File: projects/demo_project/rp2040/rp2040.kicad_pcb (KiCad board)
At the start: 2 copper layers, 30 x 60 mm, 39 parts, among them J1 1x20, J2 TC2030-IDC-NL, J3 USB_C_Receptacle_Molex_216990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, J4 1x20, SW1 PTS815, SW2 PTS815, U1 RP2040, U2 W25Q16JV, U3 TPS63051, U5 SHT40-AD1B, Y1 CSTNE12M0GH5L000R0

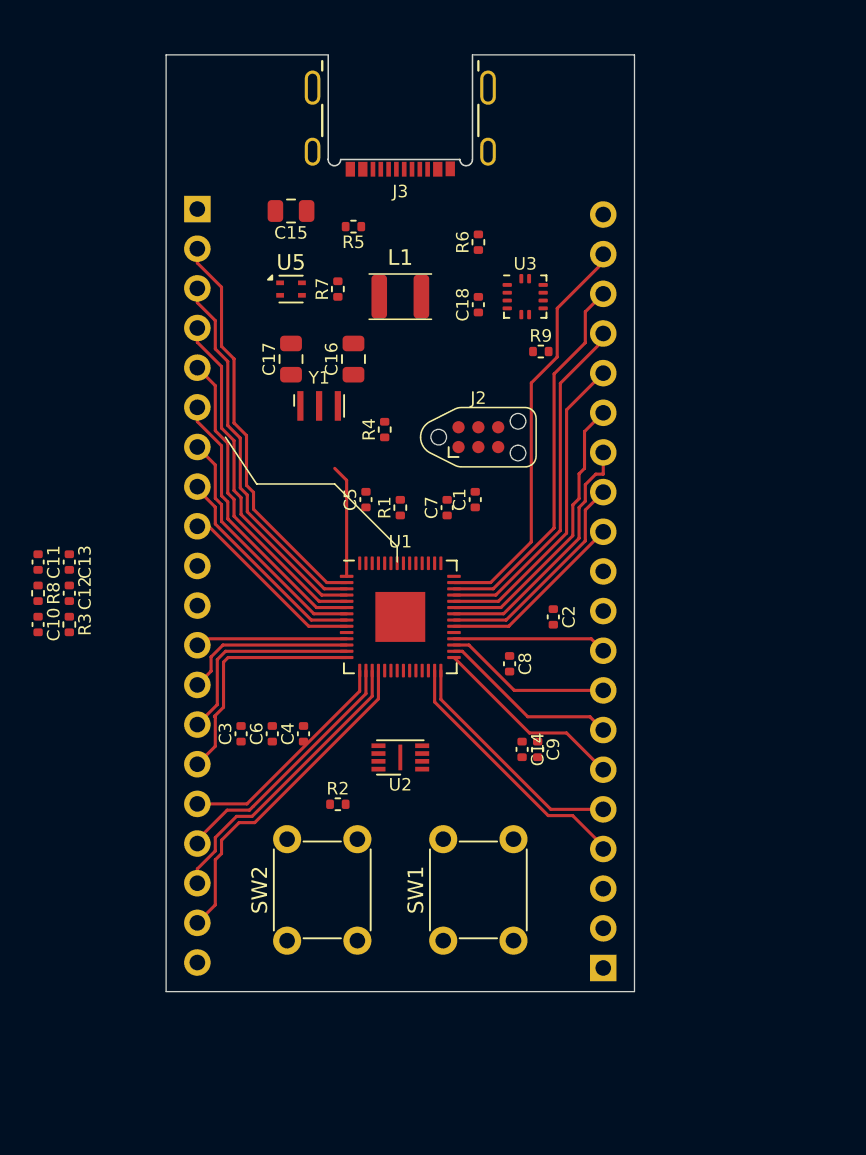
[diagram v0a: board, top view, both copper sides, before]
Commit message: rout secondary components
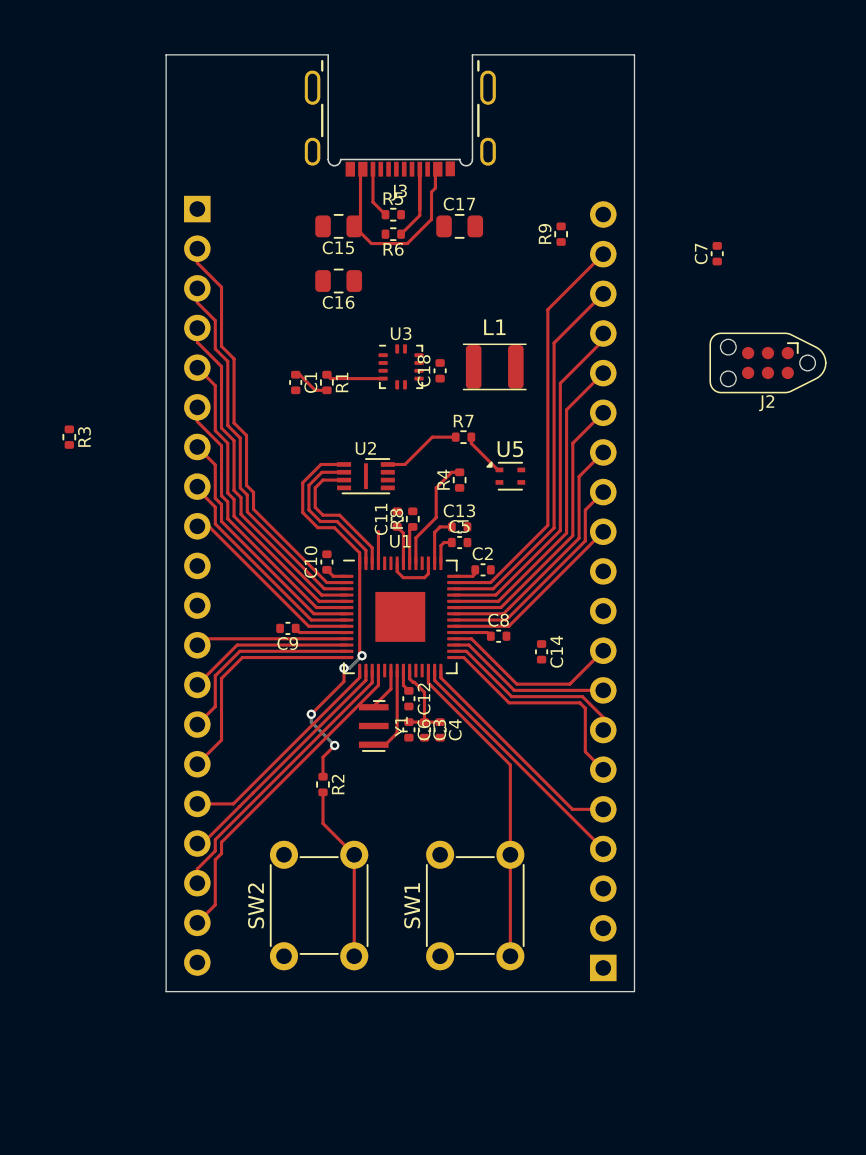
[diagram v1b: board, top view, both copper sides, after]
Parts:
- moved C13 25.1 mm to (146.0, 101.8), turned to 0 degrees
- moved R8 24.5 mm to (143.0, 101.2), turned to 90 degrees
- moved C7 23.7 mm to (162.5, 84.2)
- moved C11 23.2 mm to (142.0, 101.2), turned to 90 degrees
- moved C12 22.8 mm to (142.8, 112.8)
- moved Y1 20.8 mm to (140.5, 114.5), turned to -90 degrees
- moved J2 19.1 mm to (165.8, 91.2), turned to 180 degrees
- moved C10 18.9 mm to (137.5, 104.0), turned to 90 degrees
- moved U5 18.5 mm to (149.2, 98.5)
- moved U2 18.1 mm to (140.0, 98.5), turned to 0 degrees
- moved C9 17.8 mm to (135.0, 108.2), turned to 180 degrees
- moved C17 13.7 mm to (146.0, 82.5), turned to 0 degrees
- moved C1 13.7 mm to (135.5, 92.5), turned to -90 degrees
- moved R7 12.4 mm to (146.2, 96.0), turned to 0 degrees
- moved R3 12.0 mm to (121.0, 96.0)
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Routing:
- net Net-(U1-SPI_SS_N): track 0.00 -> 26.7 mm, vias 0 -> 4
- net +3V3: track 7.23 -> 29.0 mm
- net /RESET: track 0.00 -> 20.5 mm
- net VBUS: track 0.00 -> 13.2 mm
- net Net-(R2-Pad2): track 0.00 -> 11.3 mm
- net Net-(U1-SPI_SD1): track 0.00 -> 9.72 mm
- net Net-(U1-VREG_VOUT): track 0.00 -> 9.22 mm
- net Net-(U1-SPI_SD2): track 0.00 -> 9.02 mm
- net Net-(U1-USB_DP): track 0.00 -> 7.28 mm
- net Net-(J3-CC1): track 0.00 -> 7.27 mm
- net Net-(U1-XOUT): track 0.00 -> 6.01 mm
- net Net-(J3-CC2): track 0.00 -> 3.24 mm
- net /SDA: track 0.00 -> 2.90 mm
- net Net-(U1-XIN): track 0.00 -> 2.80 mm
- net Net-(C1-Pad1): track 0.00 -> 2.41 mm
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
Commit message: finish layout
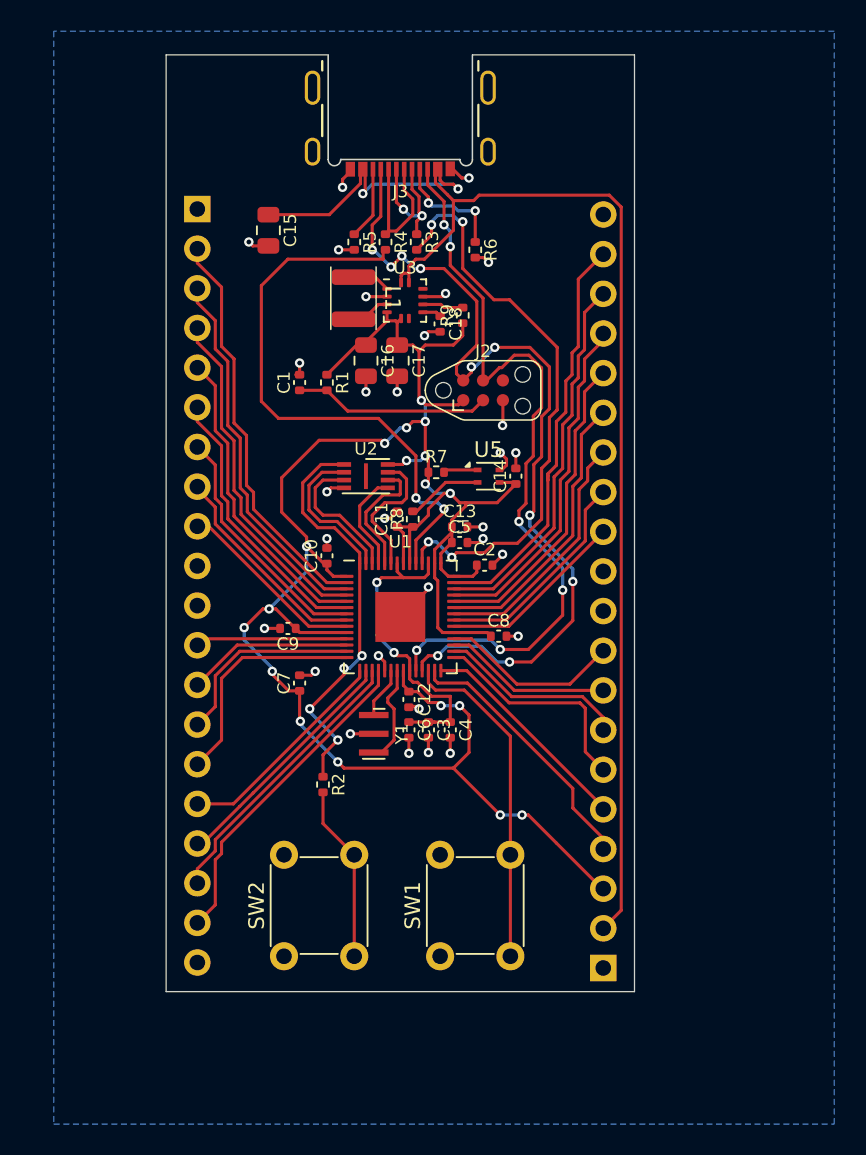
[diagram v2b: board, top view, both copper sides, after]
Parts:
- moved C7 38.4 mm to (135.8, 111.8)
- moved R3 25.5 mm to (143.2, 83.5)
- moved J2 18.3 mm to (147.5, 93.0), turned to 0 degrees
- moved R4 16.0 mm to (141.2, 83.5), turned to -90 degrees
- moved C14 11.4 mm to (149.6, 98.5), turned to 90 degrees
- moved L1 10.1 mm to (139.2, 87.1), turned to -90 degrees
- moved C17 9.48 mm to (142.0, 91.1), turned to -90 degrees
- moved R9 8.17 mm to (146.2, 88.2)
- moved C16 5.39 mm to (140.0, 91.1), turned to -90 degrees
- moved R6 5.34 mm to (147.0, 84.0), turned to -90 degrees
- moved C15 4.51 mm to (133.8, 82.8), turned to -90 degrees
- moved U3 4.26 mm to (142.5, 87.2)
- moved R5 3.05 mm to (139.2, 83.5), turned to -90 degrees
- moved C18 3.00 mm to (144.8, 88.8), turned to -90 degrees
- moved R7 2.85 mm to (144.5, 98.2)
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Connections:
- net Net-(J3-D+-PadA6) renamed /USB_P
- net Net-(J3-D--PadA7) renamed /USB_N
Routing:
- net +3V3: track 29.0 -> 138.7 mm, vias 0 -> 18
- net VBUS: track 13.2 -> 86.0 mm, vias 0 -> 2
- net /SWD_DIO: track 0.00 -> 57.1 mm, vias 0 -> 10
- net /SWD_CLK: track 0.00 -> 49.4 mm, vias 0 -> 6
- net Net-(U1-USB_DM): track 0.00 -> 38.1 mm, vias 0 -> 4
- net GND: track 0.00 -> 35.1 mm, vias 0 -> 30
- net Net-(U1-USB_DP): track 7.28 -> 36.9 mm, vias 0 -> 2
- net Net-(U1-VREG_VOUT): track 9.22 -> 20.5 mm, vias 0 -> 2
- net Net-(C1-Pad1): track 2.41 -> 12.6 mm
- net /USB_P: track 0.00 -> 9.37 mm
- net /USB_N: track 0.00 -> 8.90 mm, vias 0 -> 2
- net Net-(U1-SPI_SD3): track 0.00 -> 8.83 mm
- net Net-(U1-SPI_SCLK): track 0.00 -> 8.26 mm
- net /SCL: track 0.00 -> 4.92 mm
- net Net-(U1-SPI_SD0): track 2.03 -> 6.45 mm
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- added copper zone on B.Cu, net GND
